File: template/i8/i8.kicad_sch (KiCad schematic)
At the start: 35 parts, among them J1 ZX-SH1.0-4PWT, J2 Conn_DEBUG, SW1 MX_SW, U1 XC6206P332MR-G, U2 RP2040, U3 W25Q16JVUXIQ, Y1 Crystal_GND24

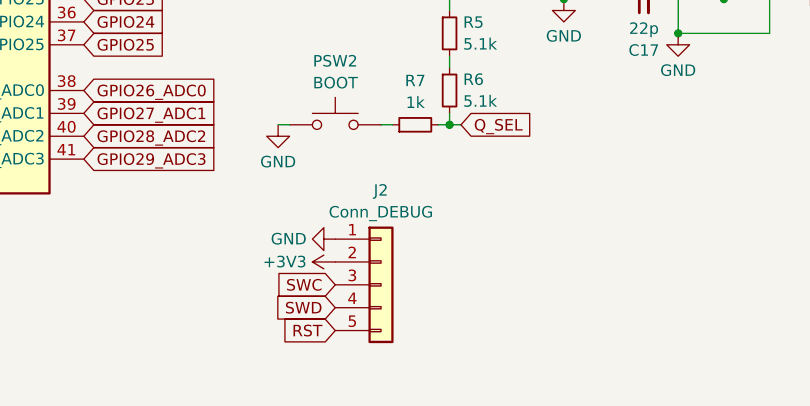
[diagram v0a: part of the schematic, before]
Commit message: i8 development
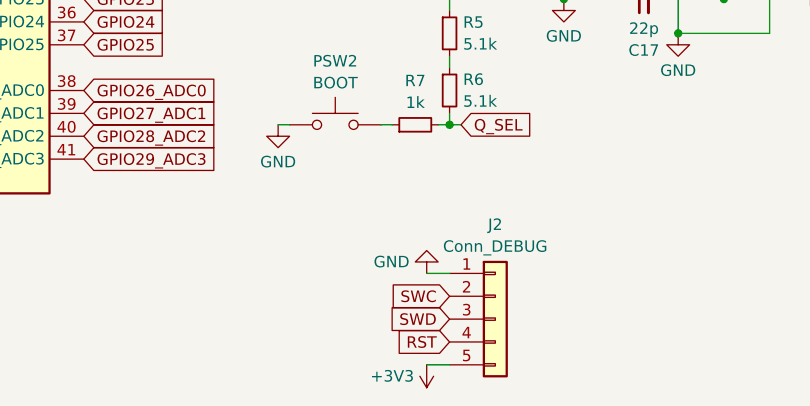
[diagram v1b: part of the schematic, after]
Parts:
- PSW1, PSW2: footprint Connector_PinHeader_1.27mm:PinHeader_1x02_P1.27mm_Vertical -> i8:JUMP_1x2
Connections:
- net +3V3: now also J2.5 (Pin_5); no longer J2.2 (Pin_2)
- net RST: now also J2.4 (Pin_4); no longer J2.5 (Pin_5)
- net SWC: now also J2.2 (Pin_2); no longer J2.3 (Pin_3)
- net SWD: now also J2.3 (Pin_3); no longer J2.4 (Pin_4)
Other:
- moved on the sheet: J2
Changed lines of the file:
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@@
 	(wire
 		(pts
+			(xy 264.16 276.86) (xy 266.7 276.86)
+		)
+		(stroke
+			(width 0)
+			(type default)
+		)
+	)
+	(wire
+		(pts
 			(xy 375.92 195.58) (xy 387.35 195.58)
 		)
@@
 	(wire
 		(pts
+			(xy 264.16 266.7) (xy 266.7 266.7)
+		)
+		(stroke
+			(width 0)
+			(type default)
+		)
+	)
+	(wire
+		(pts
 			(xy 203.2 170.18) (xy 205.74 170.18)
 		)
@@
 	(global_label "RST"
 		(shape input)
-		(at 254 273.05 180)
+		(at 266.7 274.32 180)
 		(fields_autoplaced yes)
 		(effects
@@
 		)
 		(property "Intersheetrefs" "${INTERSHEET_REFS}"
-			(at 247.5677 273.05 0)
+			(at 260.2677 274.32 0)
 			(effects
 				(font
@@
 	(global_label "SWD"
 		(shape input)
-		(at 254 270.51 180)
+		(at 266.7 271.78 180)
 		(fields_autoplaced yes)
 		(effects
@@
 		)
 		(property "Intersheetrefs" "${INTERSHEET_REFS}"
-			(at 247.0839 270.51 0)
+			(at 259.7839 271.78 0)
 			(effects
 				(font
@@
 	(global_label "SWC"
 		(shape input)
-		(at 254 267.97 180)
+		(at 266.7 269.24 180)
 		(fields_autoplaced yes)
 		(effects
@@
 		)
 		(property "Intersheetrefs" "${INTERSHEET_REFS}"
-			(at 247.0839 267.97 0)
+			(at 259.7839 269.24 0)
 			(effects
 				(font
@@
 			)
 		)
-		(property "Footprint" "Connector_PinHeader_1.27mm:PinHeader_1x02_P1.27mm_Vertical"
+		(property "Footprint" "i8:JUMP_1x2"
 			(at 254 245.11 0)
 			(effects
@@
 	(symbol
 		(lib_id "power:+3V3")
-		(at 254 265.43 90)
+		(at 264.16 276.86 0)
+		(mirror x)
 		(unit 1)
 		(exclude_from_sim no)
@@
 		(on_board yes)
 		(dnp no)
-		(fields_autoplaced yes)
 		(property "Reference" "#PWR018"
-			(at 257.81 265.43 0)
+			(at 264.16 273.05 0)
 			(effects
 				(font
@@
 		)
 		(property "Value" "+3V3"
-			(at 250.825 265.43 90)
+			(at 262.763 278.13 0)
 			(effects
 				(font
 					(size 1.27 1.27)
 				)
-				(justify left)
+				(justify right)
 			)
 		)
 		(property "Footprint" ""
-			(at 254 265.43 0)
+			(at 264.16 276.86 0)
 			(effects
 				(font
@@
 		)
 		(property "Datasheet" ""
-			(at 254 265.43 0)
+			(at 264.16 276.86 0)
 			(effects
 				(font
@@
 		)
 		(property "Description" "Power symbol creates a global label with name \"+3V3\""
-			(at 254 265.43 0)
+			(at 264.16 276.86 0)
 			(effects
 				(font
@@
 			)
 		)
-		(property "Footprint" "Connector_PinHeader_1.27mm:PinHeader_1x02_P1.27mm_Vertical"
+		(property "Footprint" "i8:JUMP_1x2"
 			(at 260.35 222.25 0)
 			(effects
@@
 	(symbol
 		(lib_id "Connector_Generic:Conn_01x05")
-		(at 259.08 267.97 0)
+		(at 271.78 271.78 0)
 		(unit 1)
 		(exclude_from_sim no)
@@
 		(dnp no)
 		(property "Reference" "J2"
-			(at 259.08 257.4755 0)
+			(at 271.78 261.2855 0)
 			(effects
 				(font
@@
 		)
 		(property "Value" "Conn_DEBUG"
-			(at 259.08 259.8998 0)
+			(at 271.78 263.7098 0)
 			(effects
 				(font
@@
 		)
 		(property "Footprint" "Connector_PinHeader_1.27mm:PinHeader_1x05_P1.27mm_Vertical"
-			(at 259.08 267.97 0)
+			(at 271.78 271.78 0)
 			(effects
 				(font
@@
 		)
 		(property "Datasheet" "~"
-			(at 259.08 267.97 0)
+			(at 271.78 271.78 0)
 			(effects
 				(font
@@
 		)
 		(property "Description" "Generic connector, single row, 01x05, script generated (kicad-library-utils/schlib/autogen/connector/)"
-			(at 259.08 267.97 0)
+			(at 271.78 271.78 0)
 			(effects
 				(font
@@
 	(symbol
 		(lib_id "power:GND")
-		(at 254 262.89 270)
+		(at 264.16 266.7 0)
 		(mirror x)
 		(unit 1)
@@
 		(fields_autoplaced yes)
 		(property "Reference" "#PWR017"
-			(at 247.65 262.89 0)
+			(at 264.16 260.35 0)
 			(effects
 				(font
@@
 		)
 		(property "Value" "GND"
-			(at 250.8251 262.89 90)
+			(at 262.2551 265.43 0)
 			(effects
 				(font
@@
 		)
 		(property "Footprint" ""
-			(at 254 262.89 0)
+			(at 264.16 266.7 0)
 			(effects
 				(font
@@
 		)
 		(property "Datasheet" ""
-			(at 254 262.89 0)
+			(at 264.16 266.7 0)
 			(effects
 				(font
@@
 		)
 		(property "Description" "Power symbol creates a global label with name \"GND\" , ground"
-			(at 254 262.89 0)
+			(at 264.16 266.7 0)
 			(effects
 				(font

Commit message: i8 development
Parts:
- C1, C10, C11, C12, C13, C14, C15, C16, C17, C2, C3, C4, C5, C6, C7, C8, C9: footprint Capacitor_SMD:C_0402_1005Metric -> i8:C_0402_1005Metric_mod
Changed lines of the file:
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@@
 			)
 		)
-		(property "Footprint" "Capacitor_SMD:C_0402_1005Metric"
+		(property "Footprint" "i8:C_0402_1005Metric_mod"
 			(at 288.29 228.6 0)
 			(effects
@@
 			)
 		)
-		(property "Footprint" "Capacitor_SMD:C_0402_1005Metric"
+		(property "Footprint" "i8:C_0402_1005Metric_mod"
 			(at 299.72 179.07 0)
 			(effects
@@
 			)
 		)
-		(property "Footprint" "Capacitor_SMD:C_0402_1005Metric"
+		(property "Footprint" "i8:C_0402_1005Metric_mod"
 			(at 325.12 198.12 0)
 			(effects
@@
 			)
 		)
-		(property "Footprint" "Capacitor_SMD:C_0402_1005Metric"
+		(property "Footprint" "i8:C_0402_1005Metric_mod"
 			(at 363.22 198.12 0)
 			(effects
@@
 			)
 		)
-		(property "Footprint" "Capacitor_SMD:C_0402_1005Metric"
+		(property "Footprint" "i8:C_0402_1005Metric_mod"
 			(at 287.02 179.07 0)
 			(effects
@@
 			)
 		)
-		(property "Footprint" "Capacitor_SMD:C_0402_1005Metric"
+		(property "Footprint" "i8:C_0402_1005Metric_mod"
 			(at 312.42 179.07 0)
 			(effects
@@
 			)
 		)
-		(property "Footprint" "Capacitor_SMD:C_0402_1005Metric"
+		(property "Footprint" "i8:C_0402_1005Metric_mod"
 			(at 287.02 198.12 0)
 			(effects
@@
 			)
 		)
-		(property "Footprint" "Capacitor_SMD:C_0402_1005Metric"
+		(property "Footprint" "i8:C_0402_1005Metric_mod"
 			(at 337.82 198.12 0)
 			(effects
@@
 			)
 		)
-		(property "Footprint" "Capacitor_SMD:C_0402_1005Metric"
+		(property "Footprint" "i8:C_0402_1005Metric_mod"
 			(at 299.72 198.12 0)
 			(effects
@@
 			)
 		)
-		(property "Footprint" "Capacitor_SMD:C_0402_1005Metric"
+		(property "Footprint" "i8:C_0402_1005Metric_mod"
 			(at 288.29 236.22 0)
 			(effects
@@
 			)
 		)
-		(property "Footprint" "Capacitor_SMD:C_0402_1005Metric"
+		(property "Footprint" "i8:C_0402_1005Metric_mod"
 			(at 312.42 198.12 0)
 			(effects
@@
 			)
 		)
-		(property "Footprint" "Capacitor_SMD:C_0402_1005Metric"
+		(property "Footprint" "i8:C_0402_1005Metric_mod"
 			(at 279.4 200.66 0)
 			(effects
@@
 			)
 		)
-		(property "Footprint" "Capacitor_SMD:C_0402_1005Metric"
+		(property "Footprint" "i8:C_0402_1005Metric_mod"
 			(at 254 200.66 0)
 			(effects
@@
 			)
 		)
-		(property "Footprint" "Capacitor_SMD:C_0402_1005Metric"
+		(property "Footprint" "i8:C_0402_1005Metric_mod"
 			(at 387.35 198.12 0)
 			(effects
@@
 			)
 		)
-		(property "Footprint" "Capacitor_SMD:C_0402_1005Metric"
+		(property "Footprint" "i8:C_0402_1005Metric_mod"
 			(at 350.52 198.12 0)
 			(effects
@@
 			)
 		)
-		(property "Footprint" "Capacitor_SMD:C_0402_1005Metric"
+		(property "Footprint" "i8:C_0402_1005Metric_mod"
 			(at 375.92 198.12 0)
 			(effects
@@
 			)
 		)
-		(property "Footprint" "Capacitor_SMD:C_0402_1005Metric"
+		(property "Footprint" "i8:C_0402_1005Metric_mod"
 			(at 370.84 222.25 0)
 			(effects

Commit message: i8 development
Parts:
- PSW1: footprint i8:JUMP_1x2 -> i8:JUMP_REST_10.16mm
- PSW2: footprint i8:JUMP_1x2 -> i8:JUMP_BOOT_10.16mm
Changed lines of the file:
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@@
 			)
 		)
-		(property "Footprint" "i8:JUMP_1x2"
+		(property "Footprint" "i8:JUMP_BOOT_10.16mm"
 			(at 254 245.11 0)
 			(effects
@@
 			)
 		)
-		(property "Footprint" "i8:JUMP_1x2"
+		(property "Footprint" "i8:JUMP_REST_10.16mm"
 			(at 260.35 222.25 0)
 			(effects
